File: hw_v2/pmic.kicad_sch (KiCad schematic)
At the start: 23 parts, among them U12 VNLD5160TR-E, U2 TC4424A, U20 VNLD5160TR-E, U3 TC4424A

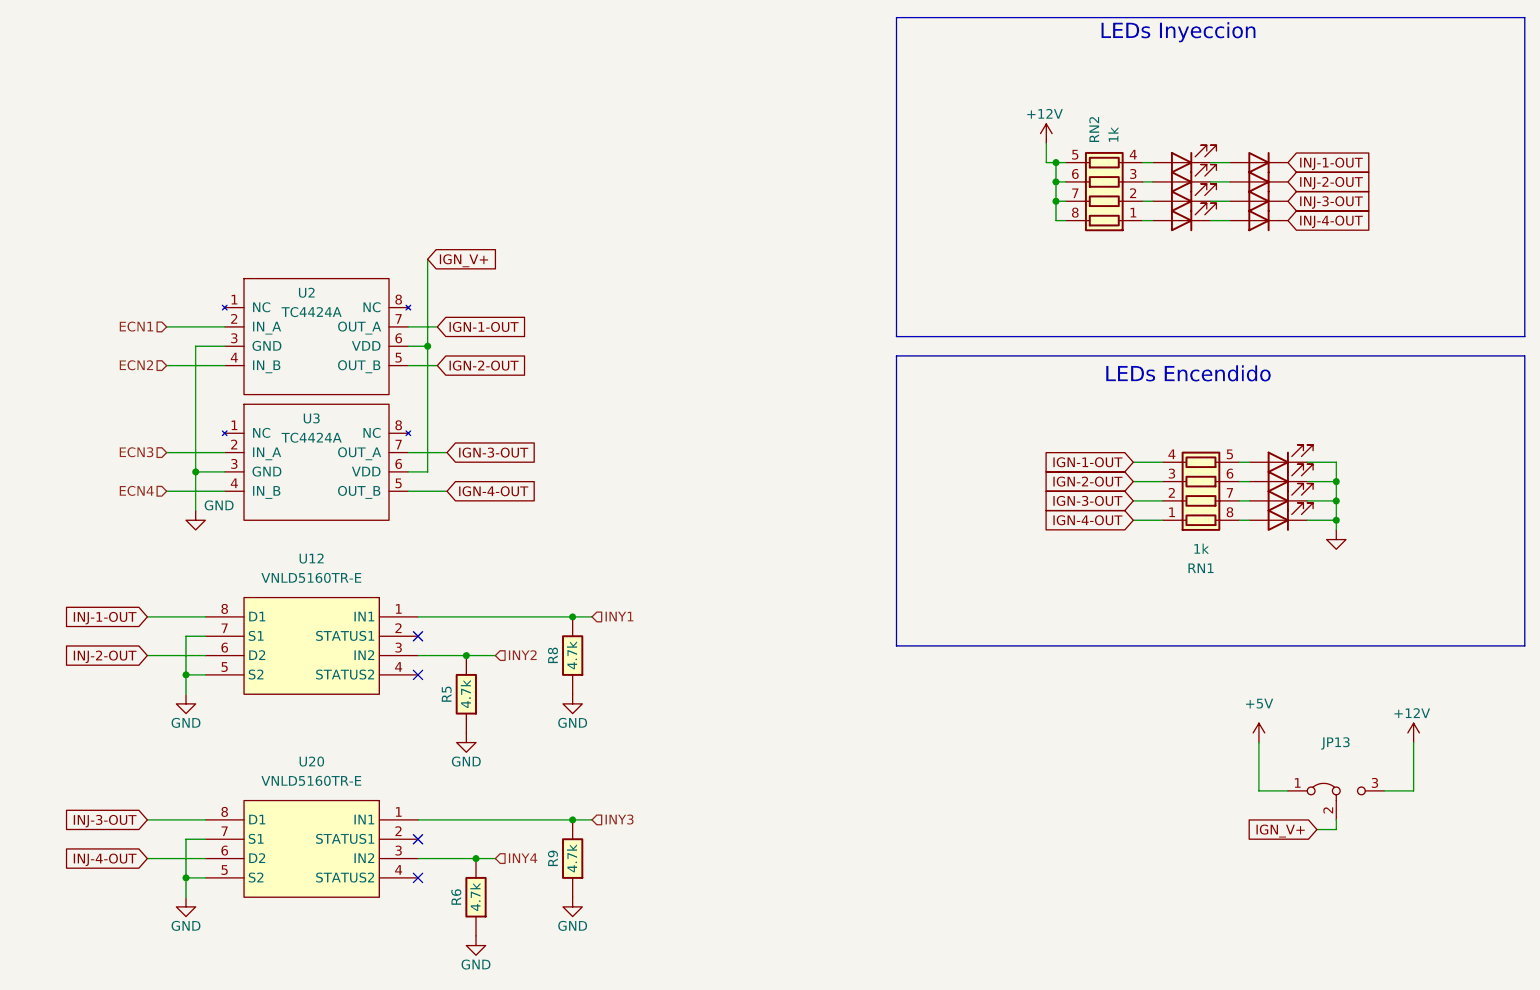
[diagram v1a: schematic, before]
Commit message: planito mas catolico
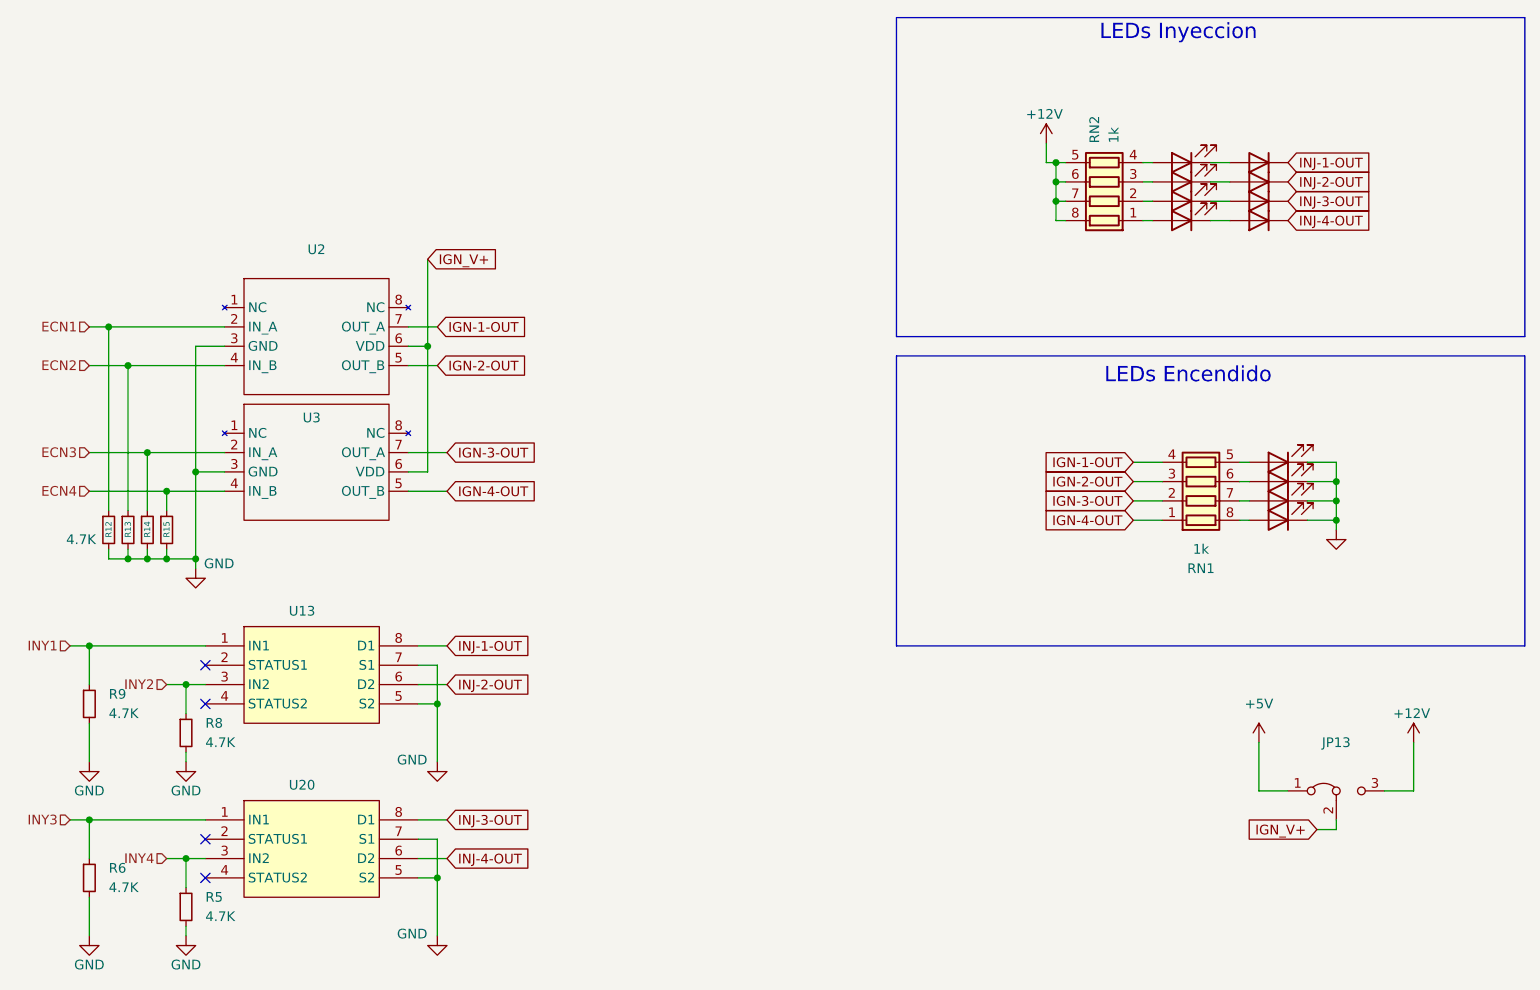
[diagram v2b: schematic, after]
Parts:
- removed R5, R6, R8, R9: 4.7k, Resistor_SMD:R_0603_1608Metric, symbol hellen-one-common:Res
- removed U12, U20: VNLD5160TR-E, Package_SO:SOIC-8_3.9x4.9mm_P1.27mm, symbol chips:VNLD5160
- removed U2, U3: TC4424A, Package_SO:SOIC-8_3.9x4.9mm_P1.27mm, symbol IC_Automotive:TC4424A
- added R12, R13, R14, R15, R5, R6, R8, R9: 4.7K, symbol Device:R_Small
- added U13, U20: ~, symbol hw_v2:VNLD5160TR-E
- added U2, U3: ~, symbol hw_v2:TC4424A
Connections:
- net ECN1: now also R12.1, U2.2 (IN_A)
- net ECN2: now also R13.1, U2.4 (IN_B)
- net ECN3: now also R14.1, U3.2 (IN_A)
- net ECN4: now also R15.1, U3.4 (IN_B)
- net GND: now also R12.2, R13.2, R14.2, R15.2, R5.2, R6.2, R8.2, R9.2, U13.5 (S2), U13.7 (S1), U2.3 (GND), U20.5 (S2), U20.7 (S1), U3.3 (GND)
- net IGN-1-OUT: now also U2.7 (OUT_A)
- net IGN-2-OUT: now also U2.5 (OUT_B)
- net IGN-3-OUT: now also U3.7 (OUT_A)
- net IGN-4-OUT: now also U3.5 (OUT_B)
- net IGN_V+: now also U2.6 (VDD), U3.6 (VDD)
- net INJ-1-OUT: now also U13.8 (D1)
- net INJ-2-OUT: now also U13.6 (D2)
- net INJ-3-OUT: now also U20.8 (D1)
- net INJ-4-OUT: now also U20.6 (D2)
- net INY1: now also R9.1, U13.1 (IN1)
- net INY2: now also R8.1, U13.3 (IN2)
- net INY3: now also R6.1, U20.1 (IN1)
- net INY4: now also R5.1, U20.3 (IN2)

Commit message: wip CKP/CMP
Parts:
- R12, R13, R14, R15, R5, R6, R8, R9: footprint (none) -> Resistor_SMD:R_0603_1608Metric
- U13, U20: footprint (none) -> Package_SO:SO-8_3.9x4.9mm_P1.27mm
- U2, U3: footprint (none) -> Package_SO:SOIC-8_3.9x4.9mm_P1.27mm
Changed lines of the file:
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@@
 (kicad_sch
-	(version 20241004)
+	(version 20241209)
 	(generator "eeschema")
 	(generator_version "8.99")
@@
 			)
 		)
-		(property "Footprint" ""
+		(property "Footprint" "Resistor_SMD:R_0603_1608Metric"
 			(at 87.63 132.08 0)
 			(effects
@@
 			)
 		)
-		(property "Footprint" ""
+		(property "Footprint" "Resistor_SMD:R_0603_1608Metric"
 			(at 100.33 135.89 0)
 			(effects
@@
 			)
 		)
-		(property "Footprint" ""
+		(property "Footprint" "Package_SO:SOIC-8_3.9x4.9mm_P1.27mm"
 			(at 116.84 68.58 0)
 			(effects
@@
 			)
 		)
-		(property "Footprint" ""
+		(property "Footprint" "Resistor_SMD:R_0603_1608Metric"
 			(at 90.17 86.36 0)
 			(effects
@@
 			)
 		)
-		(property "Footprint" ""
+		(property "Footprint" "Resistor_SMD:R_0603_1608Metric"
 			(at 87.63 109.22 0)
 			(effects
@@
 			)
 		)
-		(property "Footprint" ""
+		(property "Footprint" "Resistor_SMD:R_0603_1608Metric"
 			(at 92.71 86.36 0)
 			(effects
@@
 			)
 		)
-		(property "Footprint" ""
+		(property "Footprint" "Package_SO:SOIC-8_3.9x4.9mm_P1.27mm"
 			(at 116.84 52.07 0)
 			(effects
@@
 			)
 		)
-		(property "Footprint" ""
+		(property "Footprint" "Resistor_SMD:R_0603_1608Metric"
 			(at 100.33 113.03 0)
 			(effects
@@
 			)
 		)
-		(property "Footprint" ""
+		(property "Footprint" "Resistor_SMD:R_0603_1608Metric"
 			(at 95.25 86.36 0)
 			(effects
@@
 			)
 		)
-		(property "Footprint" ""
+		(property "Footprint" "Package_SO:SO-8_3.9x4.9mm_P1.27mm"
 			(at 115.57 105.41 0)
 			(effects
@@
 			)
 		)
-		(property "Footprint" ""
+		(property "Footprint" "Resistor_SMD:R_0603_1608Metric"
 			(at 97.79 86.36 0)
 			(effects
@@
 			)
 		)
-		(property "Footprint" ""
+		(property "Footprint" "Package_SO:SO-8_3.9x4.9mm_P1.27mm"
 			(at 115.57 128.27 0)
 			(effects
